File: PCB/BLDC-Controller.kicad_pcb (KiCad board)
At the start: 2 copper layers, 13 parts, among them J1 TC2030-NL, Q1 TPHR8504PL, Q2 TPHR8504PL, Q3 TPHR8504PL, Q4 TPHR8504PL, Q5 TPHR8504PL, Q6 TPHR8504PL, U1 UCC27282, U2 INA180A3, U3 UCC27282, U4 STM32F051K6Ux, U5 UCC27282, U6 TPS62933

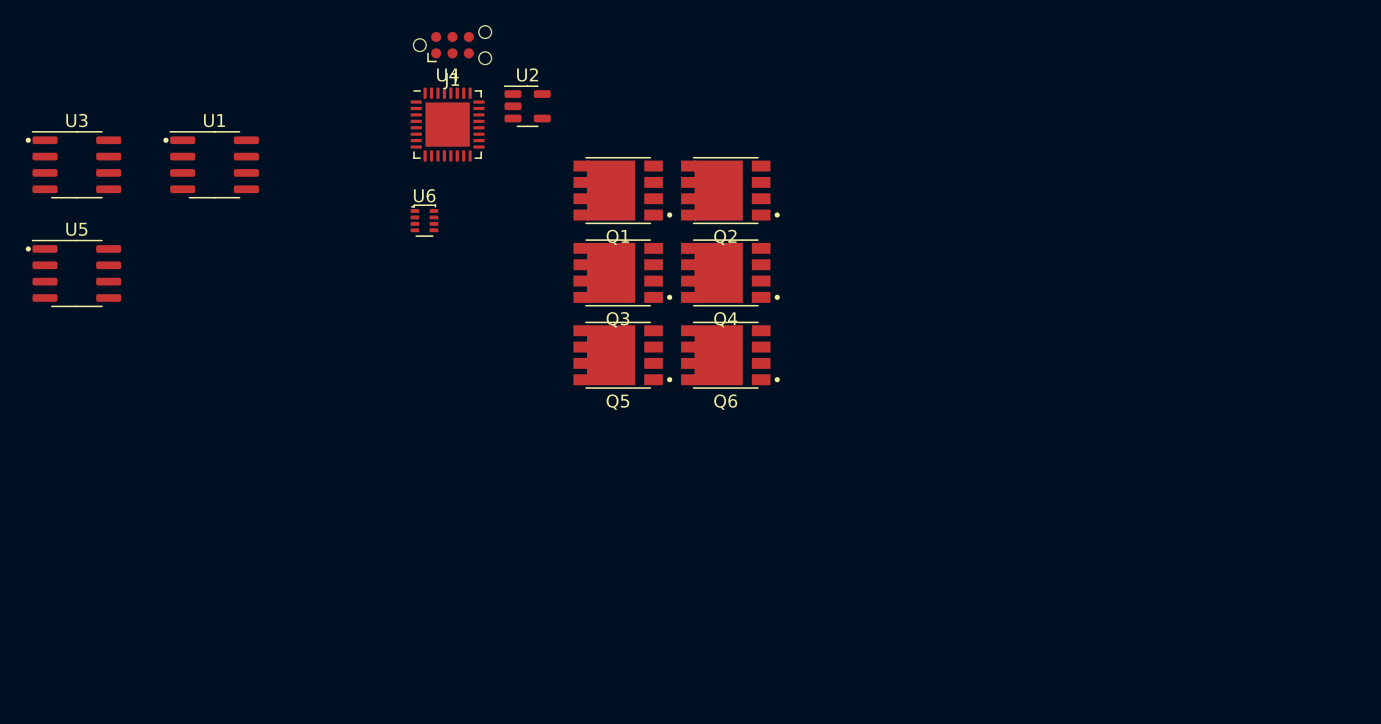
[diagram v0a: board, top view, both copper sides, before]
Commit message: d
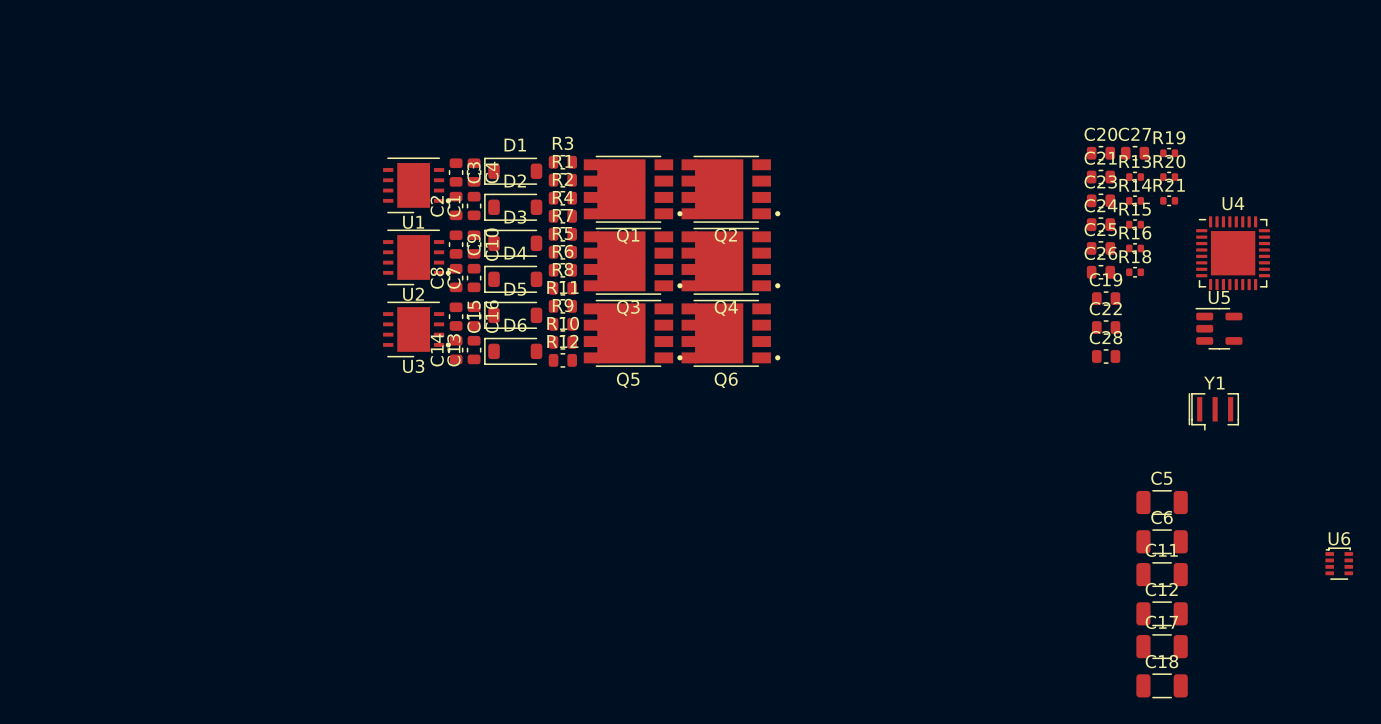
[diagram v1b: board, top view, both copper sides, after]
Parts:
- removed J1: TC2030-NL, Connector:Tag-Connect_TC2030-IDC-NL_2x03_P1.27mm_Vertical
- added C1: 1u, Ariamelon-Device:C_0603_1608Metric, F.Cu at (115.5, 84.2)
- added C10: 1u, Ariamelon-Device:C_0603_1608Metric, F.Cu at (115.5, 87.2)
- added C11: 4u7, Ariamelon-Device:C_1206_3216Metric, F.Cu at (169.0, 112.8)
- added C12: 4u7, Ariamelon-Device:C_1206_3216Metric, F.Cu at (169.0, 115.9)
- added C13: 1u, Ariamelon-Device:C_0603_1608Metric, F.Cu at (115.5, 95.4)
- added C14: 100n, Ariamelon-Device:C_0603_1608Metric, F.Cu at (114.1, 95.4)
- added C15: 1n, Ariamelon-Device:C_0603_1608Metric, F.Cu at (114.1, 92.8)
- added C16: 1u, Ariamelon-Device:C_0603_1608Metric, F.Cu at (115.5, 92.8)
- added C17: 4u7, Ariamelon-Device:C_1206_3216Metric, F.Cu at (169.0, 118.5)
- added C18: 4u7, Ariamelon-Device:C_1206_3216Metric, F.Cu at (169.0, 121.5)
- added C19: 4u7, Ariamelon-Device:C_0603_1608Metric, F.Cu at (164.6, 91.4)
- added C2: 100n, Ariamelon-Device:C_0603_1608Metric, F.Cu at (114.1, 84.2)
- added C20: 100n, Ariamelon-Device:C_0603_1608Metric, F.Cu at (164.2, 80.1)
- added C21: 100n, Ariamelon-Device:C_0603_1608Metric, F.Cu at (164.2, 82.0)
- added C22: 4u7, Ariamelon-Device:C_0603_1608Metric, F.Cu at (164.6, 93.7)
- added C23: 10n, Ariamelon-Device:C_0603_1608Metric, F.Cu at (164.2, 83.8)
- added C24: 100p, Ariamelon-Device:C_0603_1608Metric, F.Cu at (164.2, 85.7)
- added C25: 100p, Ariamelon-Device:C_0603_1608Metric, F.Cu at (164.2, 87.5)
- added C26: 100p, Ariamelon-Device:C_0603_1608Metric, F.Cu at (164.2, 89.3)
- added C27: 100p, Ariamelon-Device:C_0603_1608Metric, F.Cu at (166.9, 80.1)
- added C28: 1u, Ariamelon-Device:C_0603_1608Metric, F.Cu at (164.6, 95.9)
- added C3: 1n, Ariamelon-Device:C_0603_1608Metric, F.Cu at (114.1, 81.6)
- added C4: 1u, Ariamelon-Device:C_0603_1608Metric, F.Cu at (115.5, 81.6)
- added C5: 4u7, Ariamelon-Device:C_1206_3216Metric, F.Cu at (169.0, 107.2)
- added C6: 4u7, Ariamelon-Device:C_1206_3216Metric, F.Cu at (169.0, 110.3)
- added C7: 1u, Ariamelon-Device:C_0603_1608Metric, F.Cu at (115.5, 89.8)
- added C8: 100n, Ariamelon-Device:C_0603_1608Metric, F.Cu at (114.1, 89.8)
- added C9: 1n, Ariamelon-Device:C_0603_1608Metric, F.Cu at (114.1, 87.2)
- added D1: 4148, Diode_SMD:D_SOD-123, F.Cu at (118.7, 81.5)
- added D2: 4148, Diode_SMD:D_SOD-123, F.Cu at (118.7, 84.3)
- added D3: 4148, Diode_SMD:D_SOD-123, F.Cu at (118.7, 87.1)
- added D4: 4148, Diode_SMD:D_SOD-123, F.Cu at (118.7, 89.9)
- added D5: 4148, Diode_SMD:D_SOD-123, F.Cu at (118.7, 92.7)
- added D6: 4148, Diode_SMD:D_SOD-123, F.Cu at (118.7, 95.5)
- added R1: 22, Ariamelon-Device:R_0603_1608Metric, F.Cu at (122.4, 82.2)
- added R10: 22, Ariamelon-Device:R_0603_1608Metric, F.Cu at (122.4, 94.8)
- added R11: 10, Ariamelon-Device:R_0603_1608Metric, F.Cu at (122.4, 92.0)
- added R12: 10, Ariamelon-Device:R_0603_1608Metric, F.Cu at (122.4, 96.2)
- added R13: 10k, Ariamelon-Device:R_0402_1005Metric, F.Cu at (166.9, 82.0)
- added R14: 10k, Ariamelon-Device:R_0402_1005Metric, F.Cu at (166.9, 83.8)
- added R15: 10k, Ariamelon-Device:R_0402_1005Metric, F.Cu at (166.9, 85.7)
- added R16: 1k5, Ariamelon-Device:R_0402_1005Metric, F.Cu at (166.9, 87.5)
- added R18: 1k5, Ariamelon-Device:R_0402_1005Metric, F.Cu at (166.9, 89.3)
- added R19: 10k, Ariamelon-Device:R_0402_1005Metric, F.Cu at (169.5, 80.1)
- added R2: 22, Ariamelon-Device:R_0603_1608Metric, F.Cu at (122.4, 83.6)
- added R20: 1k5, Ariamelon-Device:R_0402_1005Metric, F.Cu at (169.5, 82.0)
- added R21: 220, Ariamelon-Device:R_0402_1005Metric, F.Cu at (169.5, 83.8)
- added R3: 10, Ariamelon-Device:R_0603_1608Metric, F.Cu at (122.4, 80.8)
- added R4: 10, Ariamelon-Device:R_0603_1608Metric, F.Cu at (122.4, 85.0)
- added R5: 22, Ariamelon-Device:R_0603_1608Metric, F.Cu at (122.4, 87.8)
- added R6: 22, Ariamelon-Device:R_0603_1608Metric, F.Cu at (122.4, 89.2)
- added R7: 10, Ariamelon-Device:R_0603_1608Metric, F.Cu at (122.4, 86.4)
- added R8: 10, Ariamelon-Device:R_0603_1608Metric, F.Cu at (122.4, 90.6)
- added R9: 22, Ariamelon-Device:R_0603_1608Metric, F.Cu at (122.4, 93.4)
- added Y1: 8M, Crystal:Resonator_SMD_Murata_CSTxExxV-3Pin_3.0x1.1mm, F.Cu at (173.1, 100.0)
- U1, U3: value UCC27282 -> UCC27282DRM; footprint Ariamelon-Package:SOIC-8_3.9x4.9mm_P1.27mm -> Ariamelon-Package:Texas_S-PVSON-N8-1EP_4x4mm_P0.8_EP2.5x3.4mm
- U2: value INA180A3 -> UCC27282DRM; footprint Package_TO_SOT_SMD:SOT-23-5 -> Ariamelon-Package:Texas_S-PVSON-N8-1EP_4x4mm_P0.8_EP2.5x3.4mm
- U5: value UCC27282 -> INA180A3; footprint Ariamelon-Package:SOIC-8_3.9x4.9mm_P1.27mm -> Package_TO_SOT_SMD:SOT-23-5
- moved U5 88.9 mm to (173.4, 93.7)
- moved U6 75.9 mm to (182.7, 112.0)
- moved U4 61.9 mm to (174.5, 87.9)
- moved U3 29.1 mm to (110.8, 93.8), turned to 180 degrees
- moved U1 15.6 mm to (110.8, 82.6), turned to 180 degrees
- moved U2 14.7 mm to (110.8, 88.2), turned to 180 degrees
- moved Q5 1.88 mm to (127.5, 94.1)
- moved Q6 1.70 mm to (135.1, 94.1)
- moved Q3 1.20 mm to (127.5, 88.5)
- moved Q4 0.90 mm to (135.1, 88.5)
- moved Q1 0.81 mm to (127.5, 82.9)
- moved Q2 0.11 mm to (135.1, 82.9)
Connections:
- U2 pad 2: GND -> Net-(U2-HB)
- U2 pad 3: GNDREF -> Net-(D3-K)
- U2 pad 4: GND -> /MCU/Phase_Out_B
- U2 pad 5: +3V3_REF -> /MCU/HI_B
- U3 pad 4: /MCU/Phase_Out_B -> /MCU/Phase_Out_C
- U3 pad 5: /MCU/HI_B -> /MCU/HI_C
- U3 pad 6: /MCU/LI_B -> /MCU/LI_C
- U4 pad 10: V_Sen_B -> V_Sen_A
- U4 pad 11: V_Sen_A -> V_Sen_B
- U4 pad 12: unconnected-(U4-PA6-Pad12) -> V_Sen_A
- U4 pad 2: unconnected-(U4-PF0-Pad2) -> Net-(U4-PF0)
- U4 pad 27: /MCU/PWM_In -> unconnected-(U4-PB4-Pad27)
- U4 pad 3: unconnected-(U4-PF1-Pad3) -> Net-(U4-PF1)
- U4 pad 6: V_Sen_C -> unconnected-(U4-PA0-Pad6)
- U4 pad 7: V_Sen_Com -> unconnected-(U4-PA1-Pad7)
- U4 pad 8: I_Sen -> /MCU/PWM_In
- U4 pad 9: unconnected-(U4-PA3-Pad9) -> I_Sen
- U5 pad 2: Net-(U5-HB) -> GND
- U5 pad 3: Net-(D5-K) (its old number) -> GNDREF
- U5 pad 4: /MCU/Phase_Out_C -> GND
- U5 pad 5: /MCU/HI_C -> +3V3_REF

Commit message: f
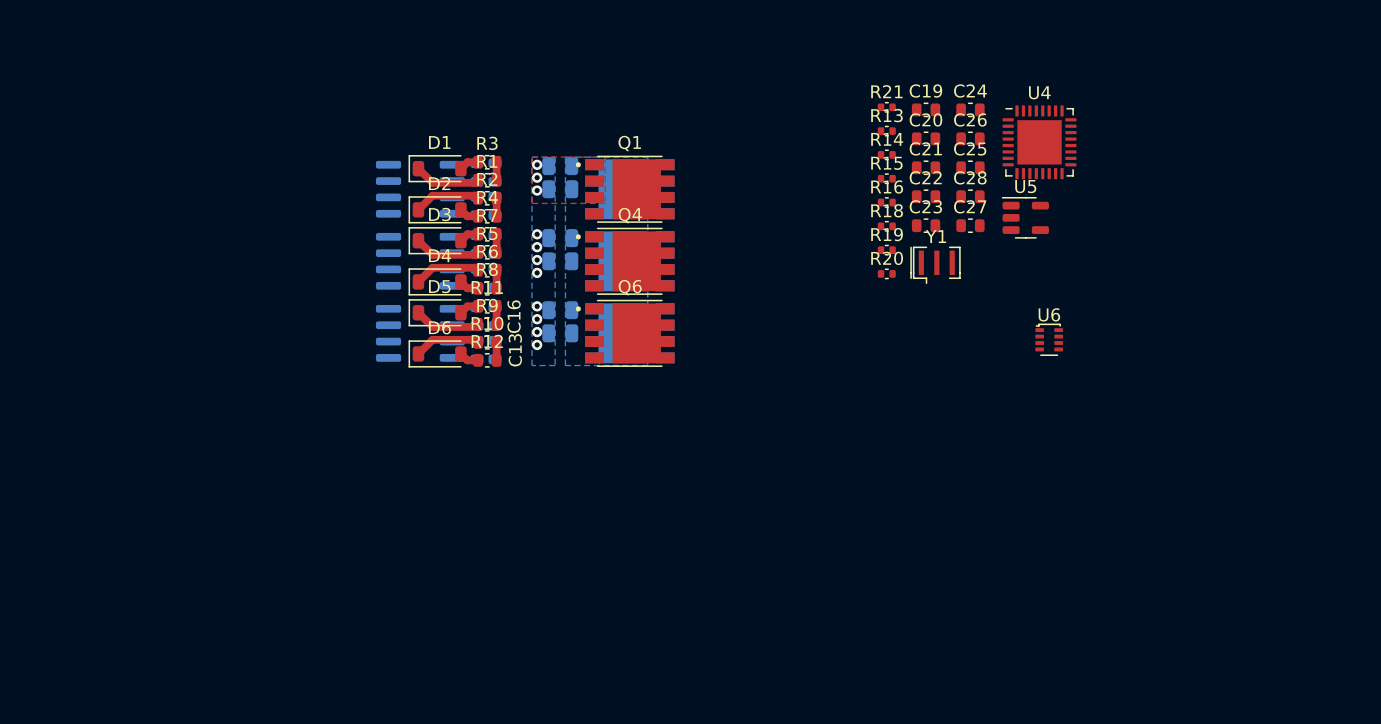
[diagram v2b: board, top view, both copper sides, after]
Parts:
- C1, C10, C13, C16, C4, C7, Q1, Q3, Q5: moved to B.Cu
- C11, C12, C17, C18, C5, C6: footprint Ariamelon-Device:C_1206_3216Metric -> Ariamelon-Device:C_0805_2012Metric; moved to B.Cu
- C14, C2, C8: value 100n -> 10n; moved to B.Cu
- C15, C3, C9: value 1n -> 10n; moved to B.Cu
- C22: value 4u7 -> 1u
- U1, U2, U3: footprint Ariamelon-Package:Texas_S-PVSON-N8-1EP_4x4mm_P0.8_EP2.5x3.4mm -> Ariamelon-Package:SOIC-8_3.9x4.9mm_P1.27mm; moved to B.Cu
- moved C12 54.2 mm to (122.2, 88.5)
- moved C18 54.2 mm to (122.2, 94.1)
- moved C6 54.2 mm to (122.2, 82.9)
- moved C11 53.6 mm to (122.2, 86.7)
- moved C17 53.6 mm to (122.2, 92.3)
- moved C5 53.6 mm to (122.2, 81.1)
- moved U6 28.5 mm to (160.2, 94.6)
- moved Y1 24.4 mm to (151.5, 88.6)
- moved R19 23.2 mm to (147.6, 87.6)
- moved R20 23.2 mm to (147.6, 89.5)
- moved R21 23.1 mm to (147.6, 76.5)
- moved C19 20.3 mm to (150.6, 76.7)
- moved R13 19.6 mm to (147.6, 78.4)
- moved R14 19.6 mm to (147.6, 80.2)
- moved R15 19.6 mm to (147.6, 82.1)
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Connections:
- net /MCU/USART_RX renamed /MCU/USART1_RX
- net /MCU/USART_TX renamed /MCU/USART1_TX
- C14 pad 1: GND -> Net-(U3-VDD)
- C14 pad 2: Net-(U3-VDD) -> GND
- C2 pad 1: GND -> Net-(U1-VDD)
- C2 pad 2: Net-(U1-VDD) -> GND
- C8 pad 1: GND -> Net-(U2-VDD)
- C8 pad 2: Net-(U2-VDD) -> GND
- U4 pad 10: V_Sen_A -> V_Sen_B
- U4 pad 11: V_Sen_B -> V_Sen_A
- U4 pad 12: V_Sen_A -> unconnected-(U4-PA6-Pad12)
- U4 pad 27: unconnected-(U4-PB4-Pad27) -> /MCU/PWM_In
- U4 pad 7: unconnected-(U4-PA1-Pad7) -> I_Sen
- U4 pad 8: /MCU/PWM_In -> V_Sen_In
- U4 pad 9: I_Sen -> V_Sen_A
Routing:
- net Net-(D6-K): track 0.00 -> 5.16 mm
- net Net-(D1-K): track 0.00 -> 5.16 mm
- net Net-(D4-K): track 0.00 -> 5.16 mm
- net Net-(D3-K): track 0.00 -> 5.16 mm
- net Net-(D5-K): track 0.00 -> 5.16 mm
- net Net-(D2-K): track 0.00 -> 5.16 mm
- net Net-(D6-A): track 0.00 -> 1.53 mm
- net Net-(D5-A): track 0.00 -> 1.53 mm
- net Net-(D4-A): track 0.00 -> 1.53 mm
- net Net-(D3-A): track 0.00 -> 1.53 mm
- net Net-(D2-A): track 0.00 -> 1.53 mm
- net Net-(D1-A): track 0.00 -> 1.53 mm
- net Net-(Q6-G): track 0.00 -> 1.40 mm
- net Net-(Q5-G): track 0.00 -> 1.40 mm
- net Net-(Q2-G): track 0.00 -> 1.40 mm
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- added copper zone on B.Cu, net GNDREF
- added copper zone on F.Cu, net GNDREF
- added copper zone on B.Cu, net VCC
